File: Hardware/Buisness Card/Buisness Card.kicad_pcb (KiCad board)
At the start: 2 copper layers, 100.7 x 62.9 mm, 35 parts, among them J101 USB_A, J102 Conn_01x03_Male, J103 Tag Connect, P1 USB_A, U101 NCP1117-12_SOT223, U102 ATtiny85-20S, U103 ProtoBoard

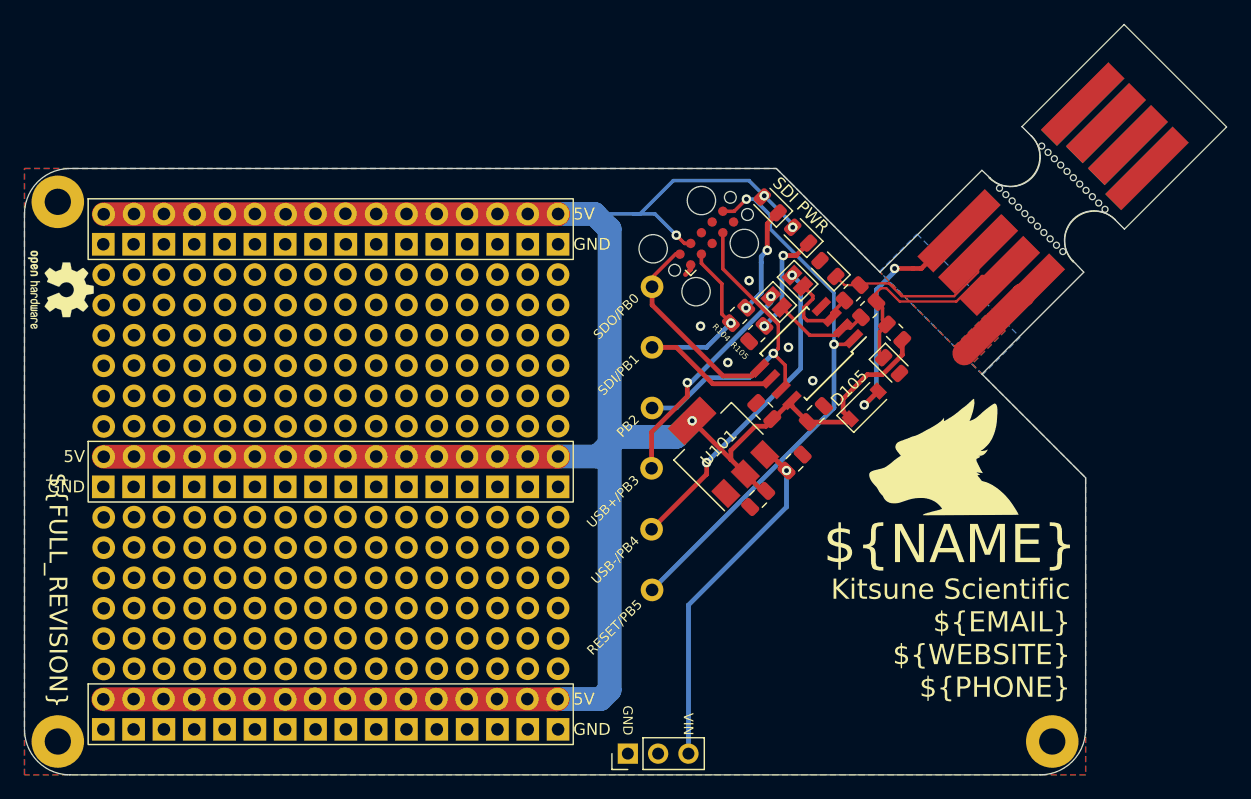
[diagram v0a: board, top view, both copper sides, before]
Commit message: Bump and make curvy
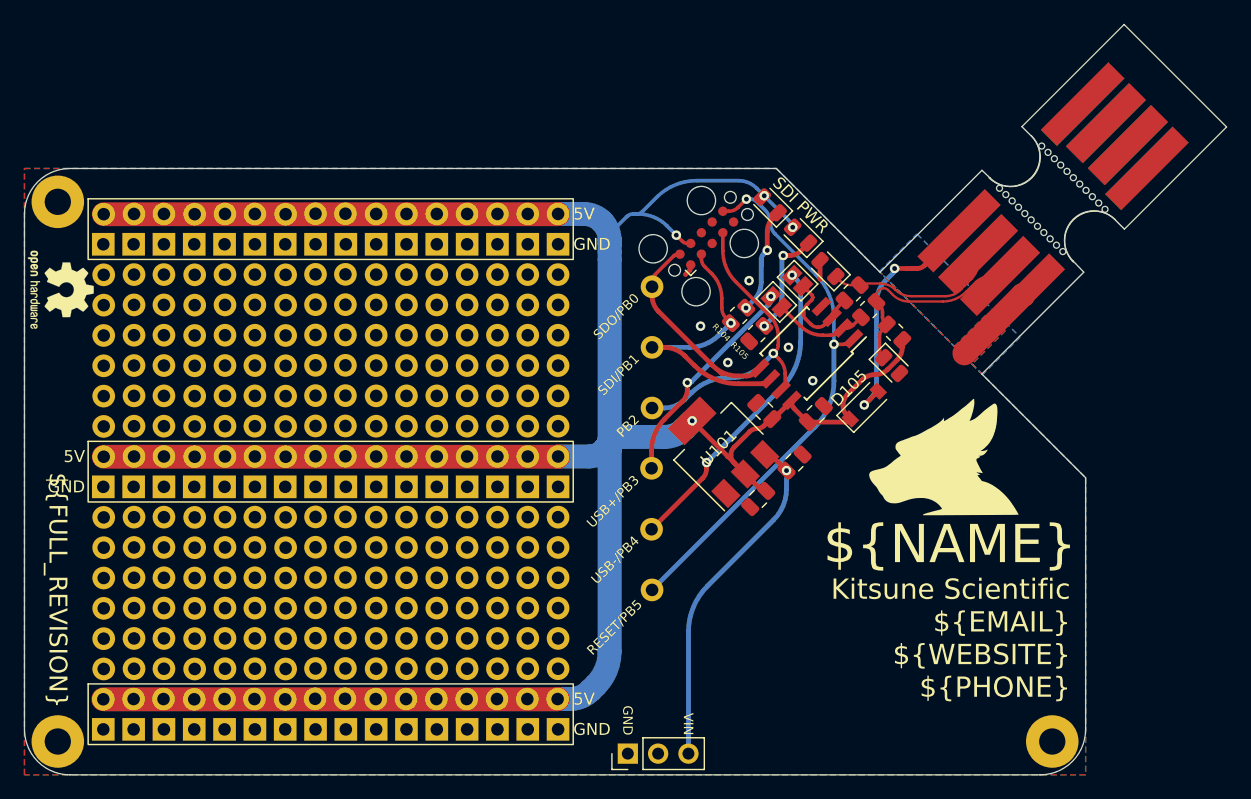
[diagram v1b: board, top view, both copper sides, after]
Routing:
- net +5V: track 232.3 -> 227.6 mm
- net /USB+: track 18.1 -> 15.0 mm
- net /SDI: track 25.6 -> 24.0 mm
- net /SCK: track 27.8 -> 26.2 mm
- net /USB-: track 15.1 -> 13.5 mm
- net GND: track 7.97 -> 9.36 mm
- net /SDO: track 25.5 -> 24.1 mm
- net Net-(C101-Pad1): track 29.5 -> 28.3 mm
- net /RST: track 46.7 -> 45.6 mm

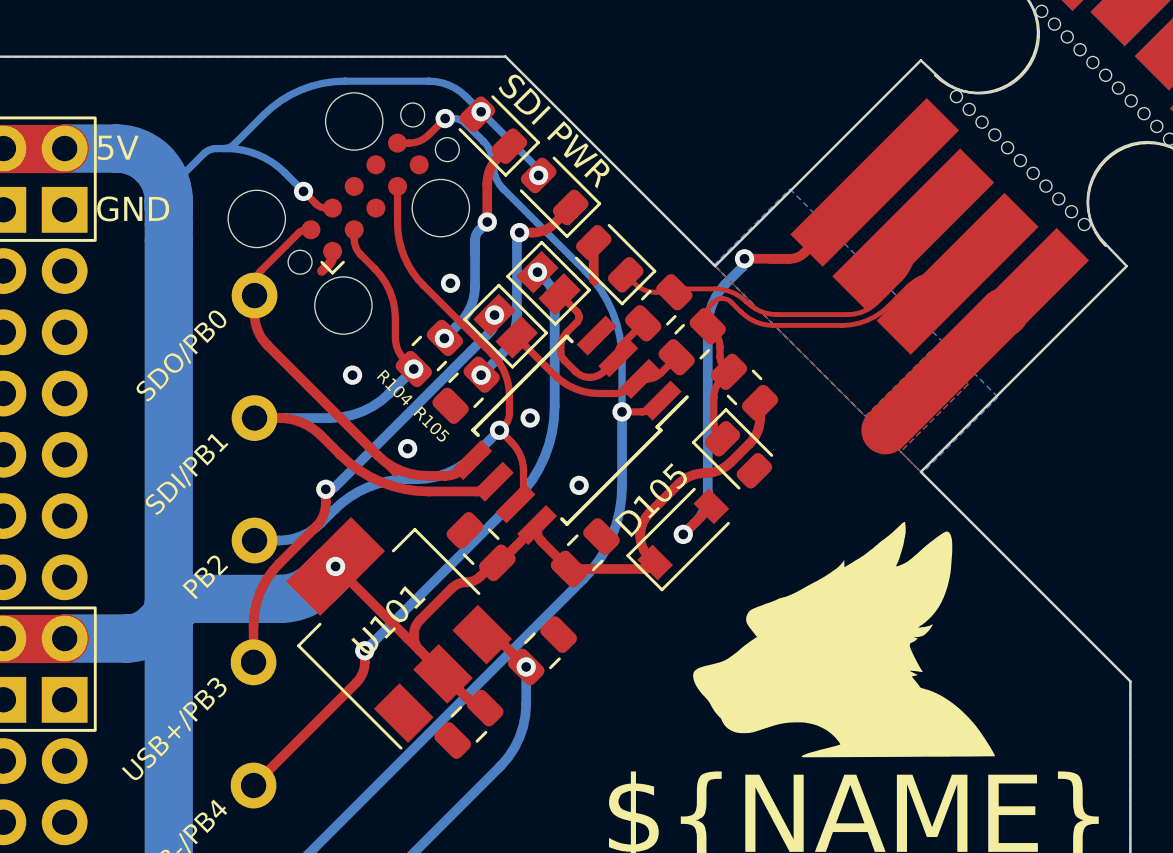
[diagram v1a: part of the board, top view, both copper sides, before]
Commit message: Prep for new order
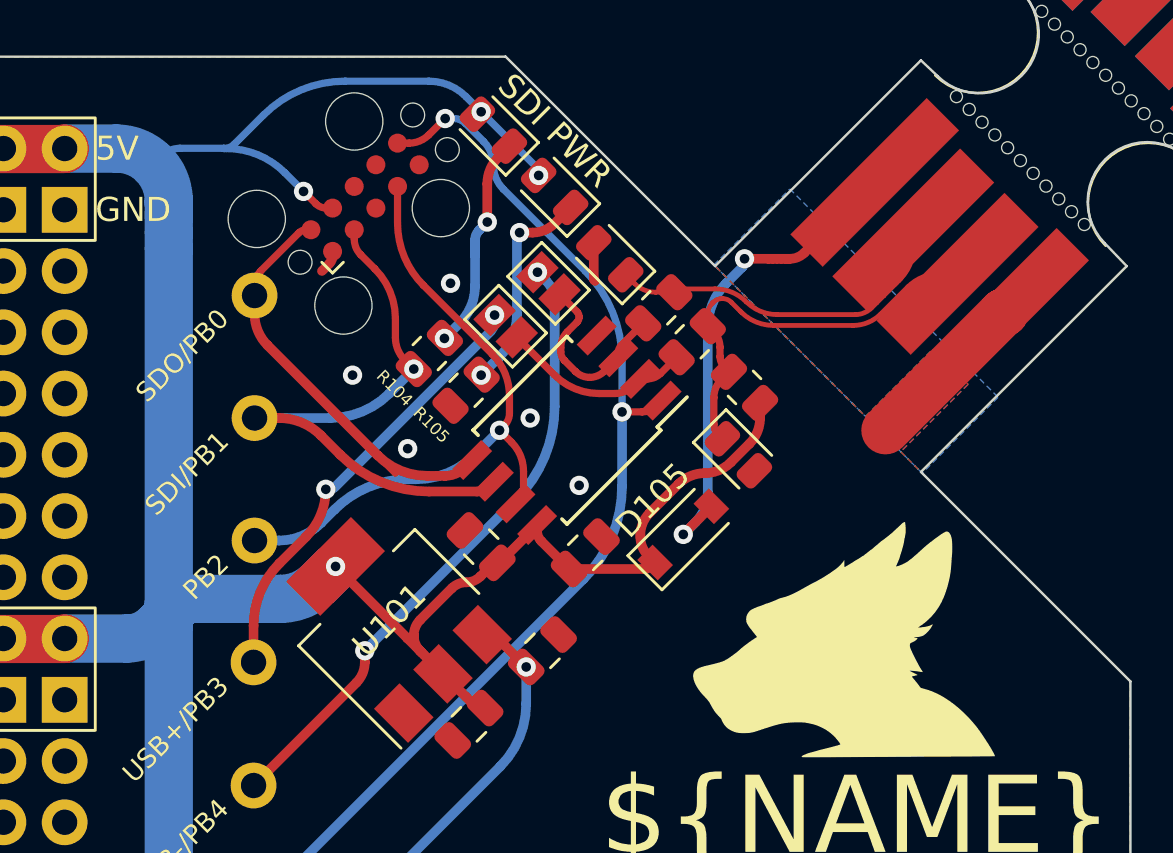
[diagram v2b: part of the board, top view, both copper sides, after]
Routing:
- net /SDO: track 24.1 -> 22.7 mm
